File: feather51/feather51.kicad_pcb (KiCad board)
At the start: 2 copper layers, 22.9 x 50.8 mm, 34 parts, among them J1 BATTERY, J2 USB_B_Micro, J3 Conn_01x12, J4 C2D, J5 Conn_01x16, SW1 RESET, U1 SPX3819M5-L-3-3, U2 EFM8UB10F16G-C-QFN28, U3 MCP73831-2-OT

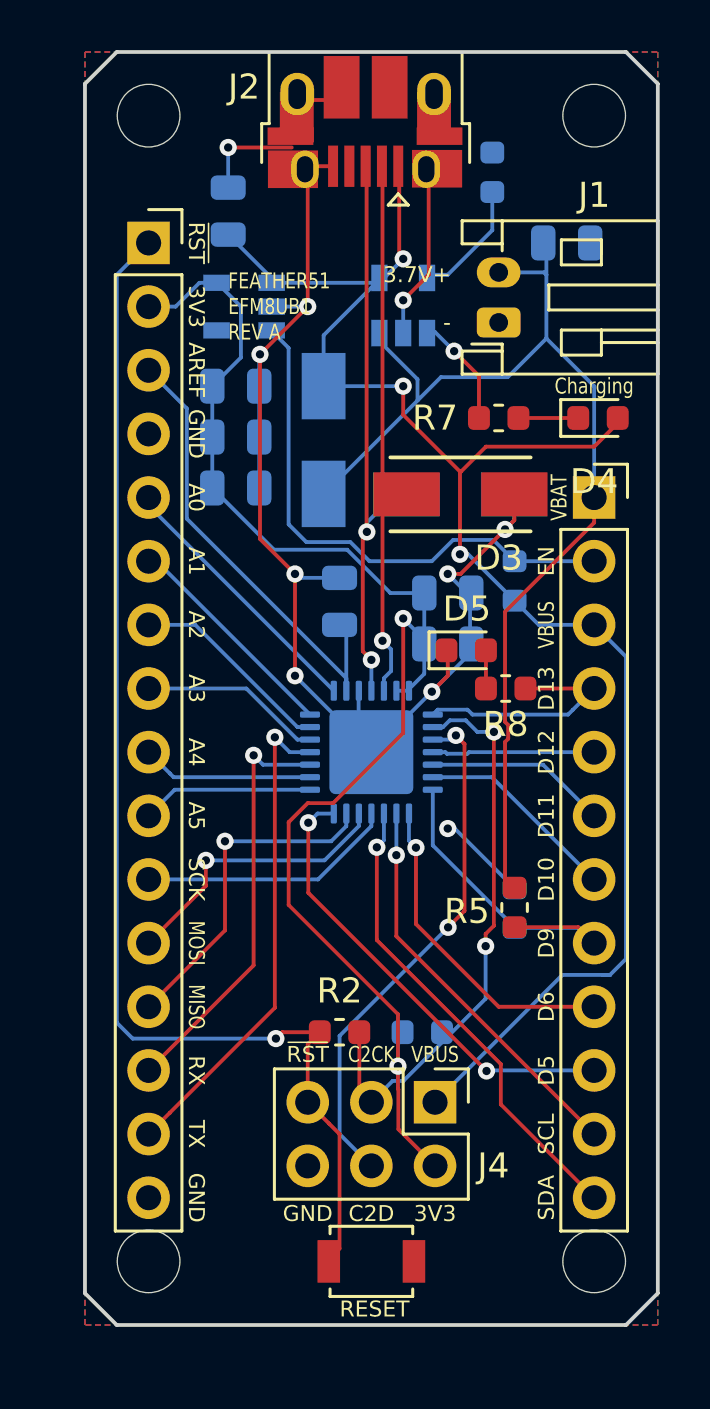
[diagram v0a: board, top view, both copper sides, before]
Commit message: Layout locked
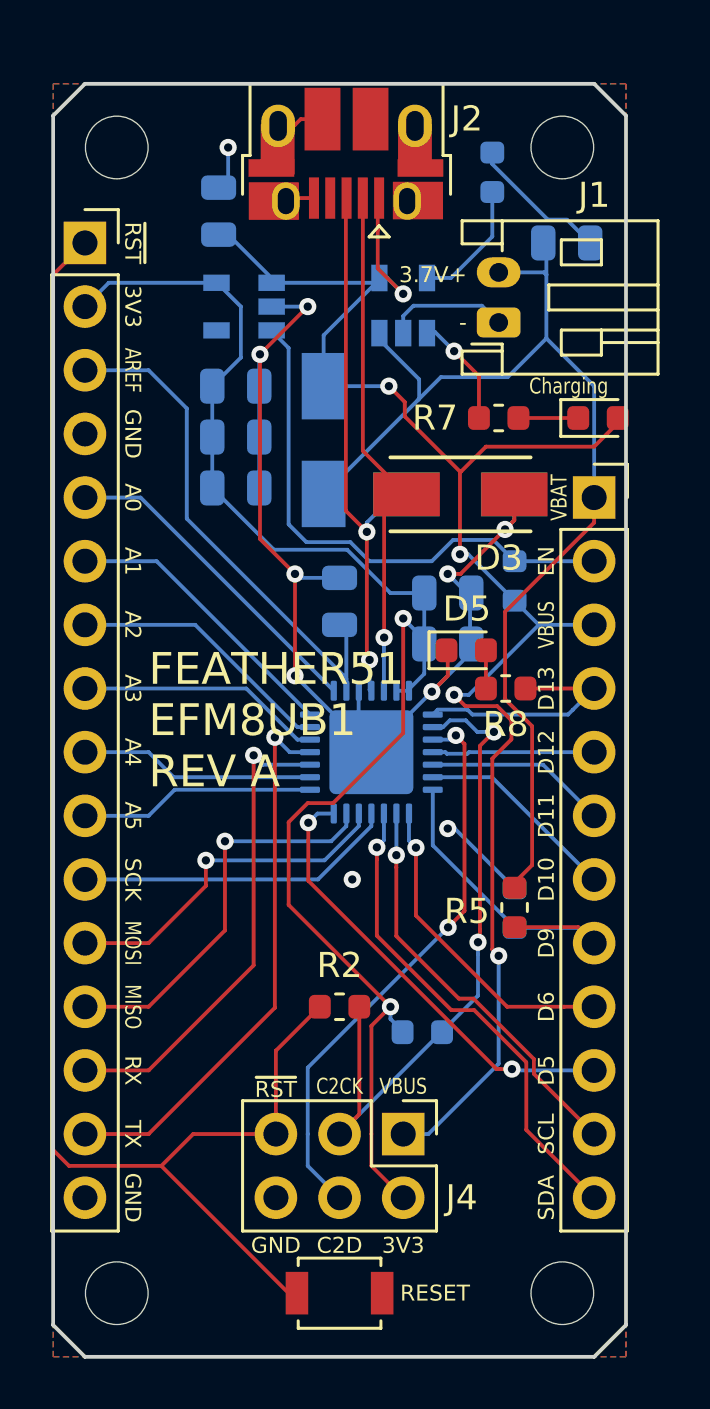
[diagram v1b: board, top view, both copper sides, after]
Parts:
- moved J5 2.54 mm to (124.5, 50.8)
- moved REF** 1.80 mm to (143.5, 47.0)
- moved J4 1.80 mm to (137.2, 86.4)
- moved REF** 1.80 mm to (143.5, 92.7)
- moved REF** 1.80 mm to (125.7, 47.0)
- moved REF** 1.80 mm to (125.7, 92.7)
- moved SW1 1.80 mm to (134.6, 92.7)
- moved J2 1.48 mm to (134.9, 47.2)
- moved R2 1.02 mm to (134.6, 81.3)
- moved C1 0.38 mm to (129.8, 49.5)
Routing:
- net /~RESET: track 50.2 -> 59.7 mm, vias 1 -> 0
- net +3V3: track 56.2 -> 60.2 mm
- net /C2CK: track 23.1 -> 27.1 mm
- net VBUS: track 65.8 -> 68.6 mm, vias 3 -> 5
- net /SCK: track 10.3 -> 12.8 mm
- net /MOSI: track 11.4 -> 14.0 mm
- net /MISO: track 13.5 -> 16.0 mm
- net /D1: track 19.6 -> 22.1 mm
- net /D0: track 16.7 -> 19.3 mm
- net /AREF: track 18.8 -> 21.3 mm
- net /A5: track 6.87 -> 9.41 mm
- net /A4: track 6.85 -> 9.39 mm
- net /A3: track 7.28 -> 9.82 mm
- net /A2: track 8.13 -> 10.7 mm
- net /A1: track 8.97 -> 11.5 mm
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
